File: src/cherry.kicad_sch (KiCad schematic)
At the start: 67 parts, among them J1 USB4085-GF-A, J2 PinHeader_1x24, J3 PinHeader_1x06, J4 PinHeader_1x06, J5 PinHeader_1x06, J6 PinHeader_1x24, SW1 RESET, SW2 USER, U1 FT2232HQ, U2 ICE40LP8K-CM81, U3 W25Q32JVSSIQ, U4 TPS62A02, U5 TPS62A02, X1 ASE-12.000MHZ-LC-T

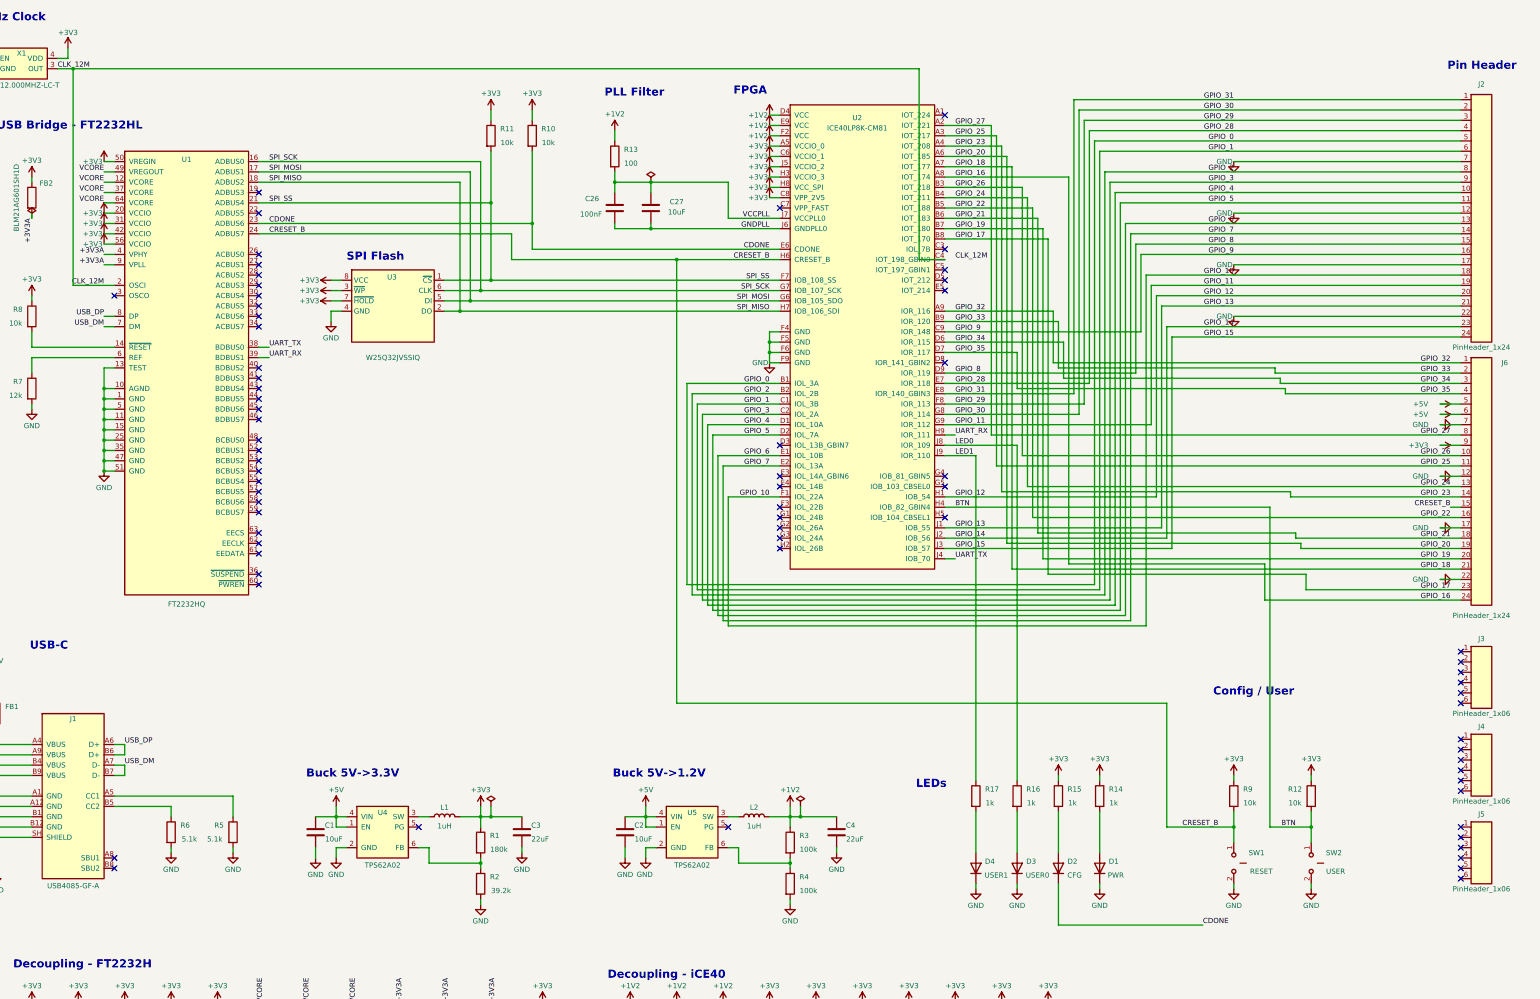
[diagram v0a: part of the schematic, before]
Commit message: wip
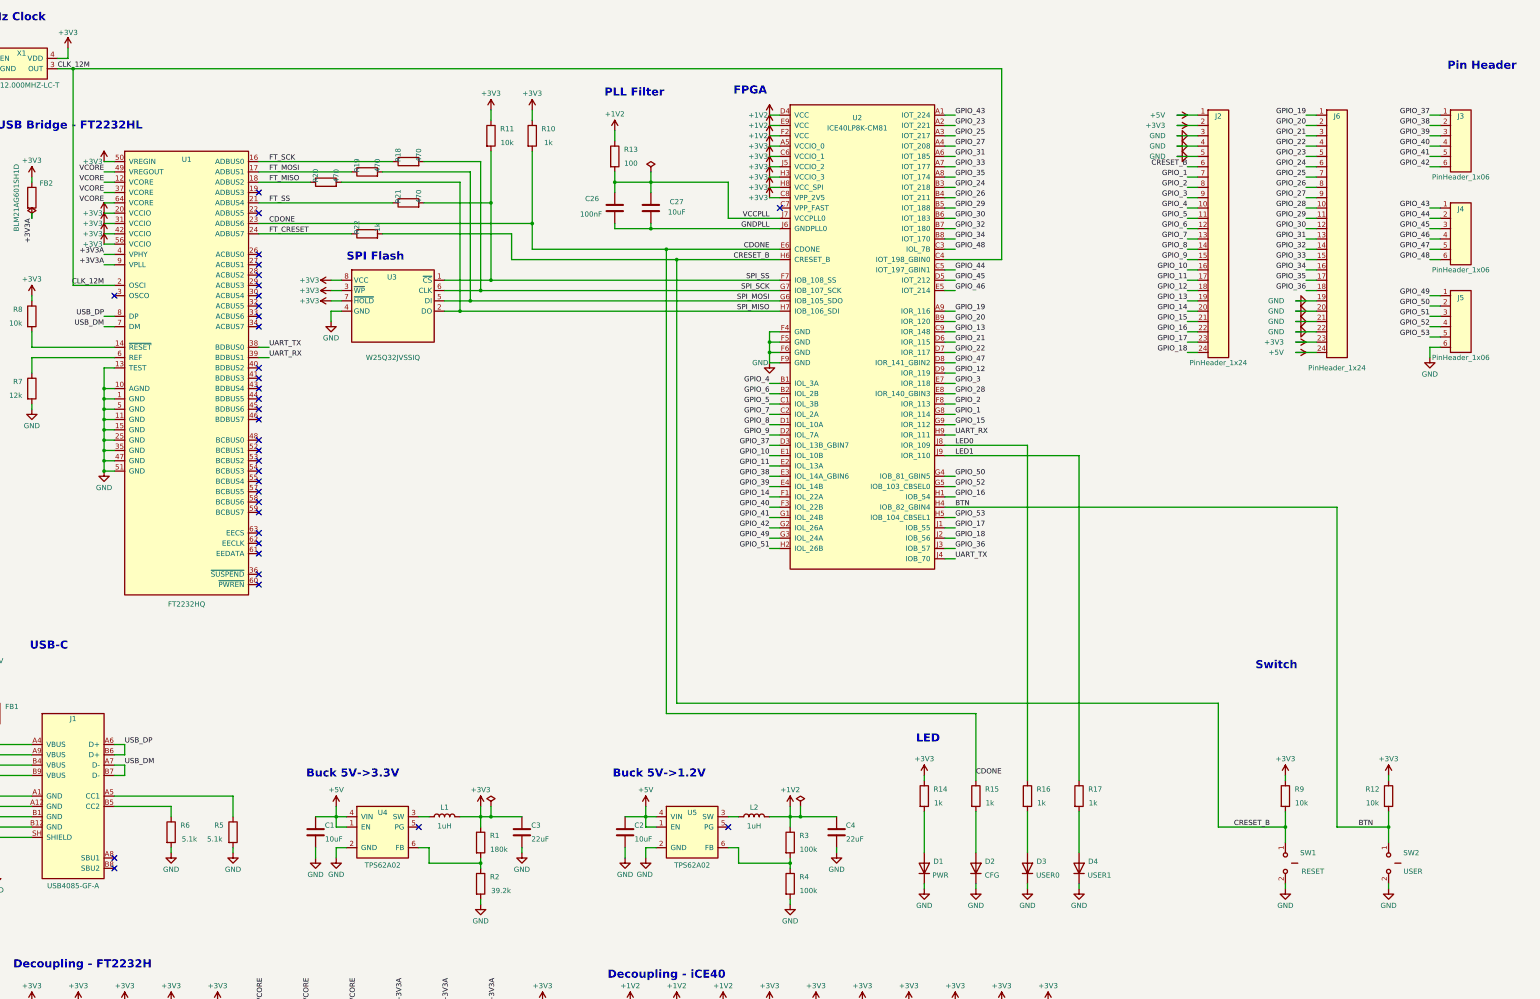
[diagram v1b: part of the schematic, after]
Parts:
- added R18, R19, R20, R21: 470, Cherry:R_0402_1005Metric, symbol Cherry:R
- added R22: 1k, Cherry:R_0402_1005Metric, symbol Cherry:R
- J2, J6: footprint Connector_PinHeader_2.54mm:PinHeader_1x24_P2.54mm_Vertical -> Cherry:PinHeader_1x24_P2.54mm
- J3, J4, J5: footprint Connector_PinHeader_2.54mm:PinHeader_1x06_P2.54mm_Vertical -> Cherry:PinHeader_1x06_P2.54mm
- R10: value 10k -> 1k
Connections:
- net +3V3: now also J2.2, J6.23; no longer J6.9, R15.1
- net +5V: now also J2.1, J6.24; no longer J6.5, J6.6
- net CDONE: now also R15.1; no longer D2.1 (K)
- net CRESET_B: now also J2.6, R22.2; no longer J6.15, U1.24 (ADBUS7)
- net GND: now also D2.1 (K), J2.3, J2.4, J2.5, J5.6 (Pin_6), J6.19, J6.20, J6.21; no longer J2.12, J2.17, J2.22, J2.7, J6.12, J6.17, J6.7
- net GPIO_1: now also J2.7, U2.G8 (IOR_114); no longer J2.6, U2.C1 (IOL_3B)
- net GPIO_10: now also J2.16, U2.E1 (IOL_10B); no longer J2.18, U2.F1 (IOL_22A)
- net GPIO_11: now also J2.17, U2.E2 (IOL_13A); no longer J2.19, U2.G9 (IOR_112)
- net GPIO_12: now also J2.18, U2.D9 (IOR_119); no longer J2.20, U2.H1 (IOB_54)
- net GPIO_13: now also J2.19, U2.C9 (IOR_148); no longer J2.21, U2.J1 (IOB_55)
- net GPIO_14: now also J2.20, U2.F1 (IOL_22A); no longer J2.23, U2.J2 (IOB_56)
- net GPIO_15: now also J2.21, U2.G9 (IOR_112); no longer J2.24, U2.J3 (IOB_57)
- net GPIO_16: now also J2.22, U2.H1 (IOB_54); no longer J6.24, U2.A8 (IOT_174)
- net GPIO_17: now also J2.23, U2.J1 (IOB_55); no longer J6.23, U2.B8 (IOT_170)
- net GPIO_18: now also J2.24, U2.J2 (IOB_56); no longer J6.21, U2.A7 (IOT_177)
- net GPIO_19: now also J6.1, U2.A9 (IOR_116); no longer J6.20, U2.B7 (IOT_180)
- net GPIO_2: now also U2.F8 (IOR_113); no longer U2.B2 (IOL_2B)
- net GPIO_20: now also J6.2, U2.B9 (IOR_120); no longer J6.19, U2.A6 (IOT_185)
- net GPIO_21: now also J6.3, U2.D6 (IOR_115); no longer J6.18, U2.B6 (IOT_183)
- net GPIO_22: now also J6.4, U2.D7 (IOR_117); no longer J6.16, U2.B5 (IOT_188)
- net GPIO_23: now also J6.5, U2.A2 (IOT_221); no longer J6.14, U2.A4 (IOT_208)
- net GPIO_24: now also J6.6, U2.B3 (IOT_218); no longer J6.13, U2.B4 (IOT_211)
- net GPIO_25: now also J6.7; no longer J6.11
- net GPIO_26: now also J6.8, U2.B4 (IOT_211); no longer J6.10, U2.B3 (IOT_218)
- net GPIO_27: now also J6.9, U2.A4 (IOT_208); no longer J6.8, U2.A2 (IOT_221)
- net GPIO_28: now also J6.10, U2.E8 (IOR_140_GBIN3); no longer J2.4, U2.E7 (IOR_118)
- net GPIO_29: now also J6.11, U2.B5 (IOT_188); no longer J2.3, U2.F8 (IOR_113)
- net GPIO_3: now also U2.E7 (IOR_118); no longer U2.C2 (IOL_2A)
- net GPIO_30: now also J6.12, U2.B6 (IOT_183); no longer J2.2, U2.G8 (IOR_114)
- net GPIO_31: now also J6.13, U2.A6 (IOT_185); no longer J2.1, U2.E8 (IOR_140_GBIN3)
- net GPIO_32: now also J6.14, U2.B7 (IOT_180); no longer J6.1, U2.A9 (IOR_116)
- net GPIO_33: now also J6.15, U2.A7 (IOT_177); no longer J6.2, U2.B9 (IOR_120)
- net GPIO_34: now also J6.16, U2.B8 (IOT_170); no longer J6.3, U2.D6 (IOR_115)
- net GPIO_35: now also J6.17, U2.A8 (IOT_174); no longer J6.4, U2.D7 (IOR_117)
- net GPIO_4: now also U2.B1 (IOL_3A); no longer U2.D1 (IOL_10A)
- net GPIO_5: now also U2.C1 (IOL_3B); no longer U2.D2 (IOL_7A)
- net GPIO_6: now also J2.12, U2.B2 (IOL_2B); no longer J2.13, U2.E1 (IOL_10B)
- net GPIO_7: now also J2.13, U2.C2 (IOL_2A); no longer J2.14, U2.E2 (IOL_13A)
- net GPIO_8: now also J2.14, U2.D1 (IOL_10A); no longer J2.15, U2.D9 (IOR_119)
- net GPIO_9: now also J2.15, U2.D2 (IOL_7A); no longer J2.16, U2.C9 (IOR_148)
- net SPI_MISO: now also R20.2; no longer U1.18 (ADBUS2)
- net SPI_MOSI: now also R19.2; no longer U1.17 (ADBUS1)
- net SPI_SCK: now also R18.2; no longer U1.16 (ADBUS0)
- net SPI_SS: now also R21.2; no longer U1.21 (ADBUS4)
- net GPIO_49: now reaches J5.1 (Pin_1)
- net GPIO_49: now also U2.G3 (IOL_24A)
- net GPIO_50: now reaches J5.2 (Pin_2)
- net GPIO_50: now also U2.G4 (IOB_81_GBIN5)
- net GPIO_51: now reaches J5.3 (Pin_3)
- net GPIO_51: now also U2.H2 (IOL_26B)
- net GPIO_52: now reaches J5.4 (Pin_4)
- net GPIO_52: now also U2.G5 (IOB_103_CBSEL0)
- net GPIO_53: now reaches J5.5 (Pin_5)
- net GPIO_53: now also U2.H5 (IOB_104_CBSEL1)
- net GPIO_43: now reaches J4.1 (Pin_1)
- net GPIO_43: now also U2.A1 (IOT_224)
- net GPIO_44: now reaches J4.2 (Pin_2)
- net GPIO_44: now also U2.C5 (IOT_197_GBIN1)
- net GPIO_45: now reaches J4.3 (Pin_3)
- net GPIO_45: now also U2.D5 (IOT_212)
- net GPIO_46: now reaches J4.4 (Pin_4)
- net GPIO_46: now also U2.E5 (IOT_214)
- net GPIO_47: now reaches J4.5 (Pin_5)
- net GPIO_47: now also U2.D8 (IOR_141_GBIN2)
- net GPIO_48: now reaches J4.6 (Pin_6)
- net GPIO_48: now also U2.C3 (IOL_7B)
- net GPIO_37: now reaches U2.D3 (IOL_13B_GBIN7)
- net GPIO_37: now also J3.1 (Pin_1)
- net GPIO_38: now reaches U2.E3 (IOL_14A_GBIN6)
- net GPIO_38: now also J3.2 (Pin_2)
- net GPIO_39: now reaches U2.E4 (IOL_14B)
- net GPIO_39: now also J3.3 (Pin_3)
- net GPIO_40: now reaches U2.F3 (IOL_22B)
- net GPIO_40: now also J3.4 (Pin_4)
- net GPIO_41: now reaches U2.G1 (IOL_24B)
- net GPIO_41: now also J3.5 (Pin_5)
- net GPIO_42: now reaches U2.G2 (IOL_26A)
- net GPIO_42: now also J3.6 (Pin_6)
- removed net GPIO_0: J2.5, U2.B1 (IOL_3A)
- new net FT_CRESET: R22.1, U1.24 (ADBUS7)
- new net FT_MISO: R20.1, U1.18 (ADBUS2)
- new net FT_MOSI: R19.1, U1.17 (ADBUS1)
- new net FT_SCK: R18.1, U1.16 (ADBUS0)
- new net FT_SS: R21.1, U1.21 (ADBUS4)
- new net GPIO_36: J6.18, U2.J3 (IOB_57)
- no-connect marks 70 -> 35
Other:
- note added: "LED"
- note added: "Switch"
- note removed: "Config / User"
- note removed: "LEDs"
- moved on the sheet: D1, D2, D3, D4, J2, J3, J4, J5, J6, R12, R14, R15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
